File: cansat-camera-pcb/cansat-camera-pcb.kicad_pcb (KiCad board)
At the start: 8 copper layers, 50 x 50 mm, 60 parts, among them IC1 W9825G6JB-6I, IC2 TLV74315PDBVR, J3 Conn_01x05_Socket, J4 Conn_02x10_Odd_Even, J5 Conn_02x10_Odd_Even, J6 OV5640, SW2 SW_Push, U2 AP2112K-3.3, U4 STM32H743ZITx, U6 TLV74328PDBVR, Y1 24MHz

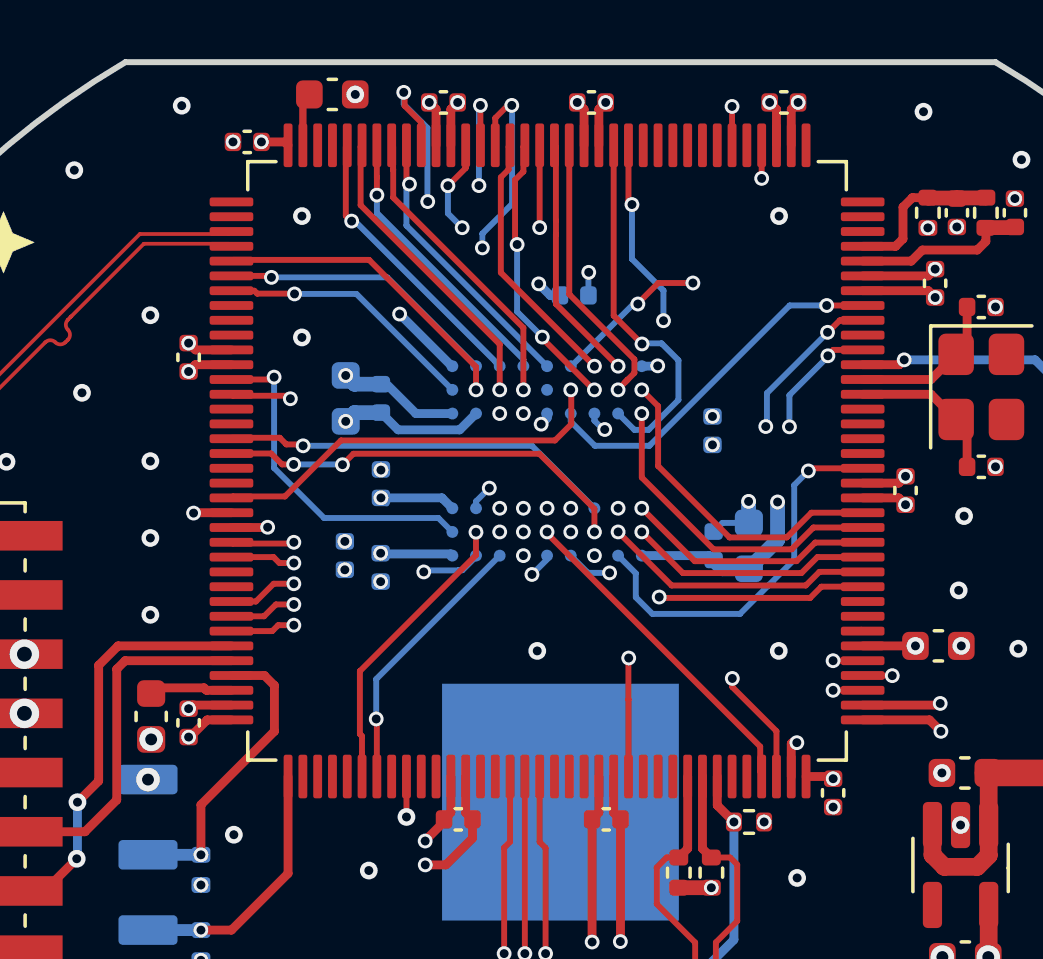
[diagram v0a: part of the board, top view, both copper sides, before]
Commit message: Sdram finish, cleanup
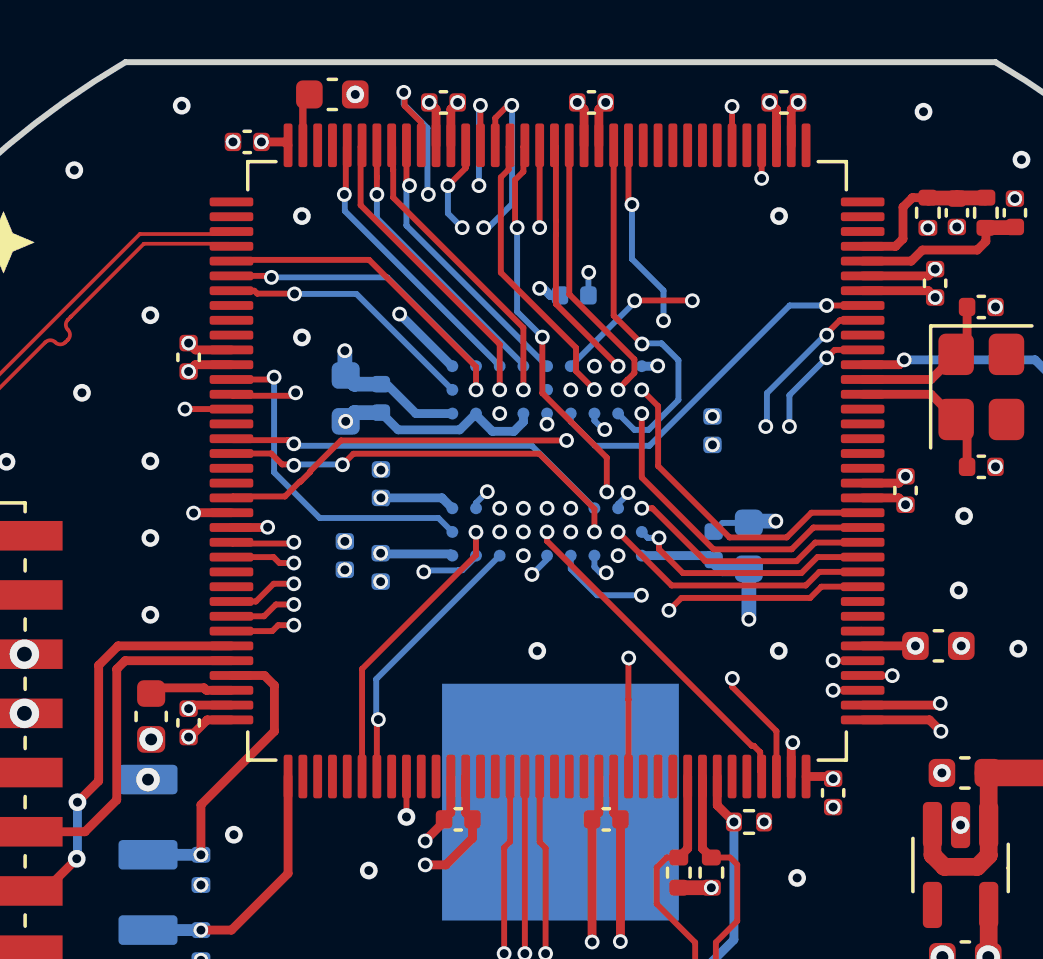
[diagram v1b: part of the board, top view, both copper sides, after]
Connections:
- IC1 pad G1: /FMC_A11 -> /FMC_A12
- IC1 pad G2: /FMC_A10 -> /FMC_A11
- IC1 pad H9: /FMC_AP -> /FMC_A10
- U4 pad 18: /FMC_AP -> unconnected-(U4-PF6-Pad18)
- U4 pad 87: unconnected-(U4-PG2-Pad87) -> /FMC_A12
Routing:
- net /FMC_A12: track 0.00 -> 16.0 mm, vias 0 -> 2
- net /FMC_AP: track 13.1 -> 0.00 mm, vias 1 -> 0
- net /FMC_A10: track 9.52 -> 16.1 mm, vias 3 -> 4
- net +3.3V: track 66.3 -> 62.4 mm, vias 37 -> 36
- net /FMC_D1: track 11.8 -> 14.0 mm
- net /FMC_SDNWE: track 13.9 -> 15.6 mm
- net /FMC_SDNE0: track 13.1 -> 14.6 mm
- net /FMC_SDNCAS: track 14.3 -> 15.7 mm
- net GND: track 38.7 -> 39.6 mm
- net /FMC_A11: track 8.90 -> 9.69 mm
- net /FMC_A0: track 12.0 -> 12.6 mm
- net /FMC_NBL1: track 23.1 -> 22.6 mm
- net /FMC_SDCLK: track 13.7 -> 13.9 mm, vias 1 -> 2

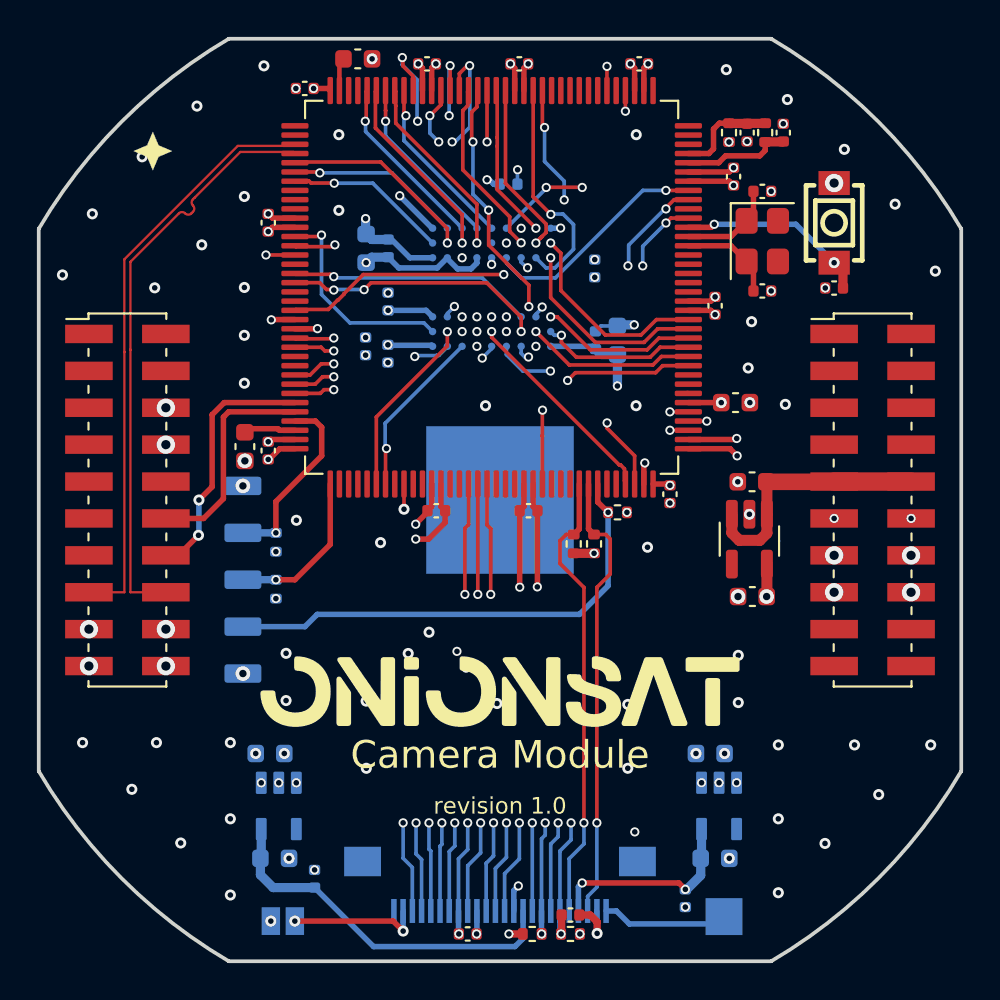
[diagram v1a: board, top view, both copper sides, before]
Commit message: Cleanup finish
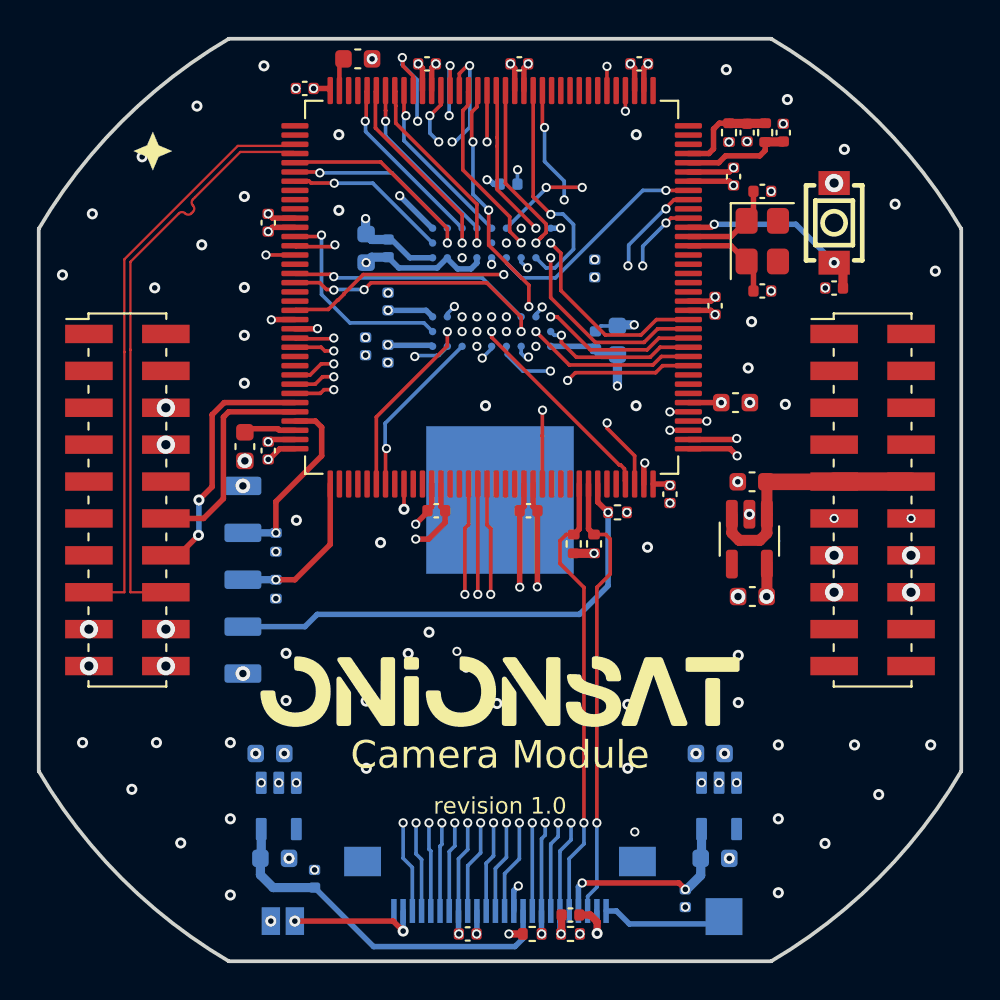
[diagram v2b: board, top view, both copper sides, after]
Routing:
- net /camera/DATA1: track 7.74 -> 7.18 mm
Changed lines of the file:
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@@
 	)
 	(segment
-		(start 68.511012 111.13)
-		(end 68.49 111.13)
-		(width 0.2)
-		(layer "B.Cu")
-		(net 1)
-	)
-	(segment
 		(start 76.672012 112.891)
 		(end 77.199 112.891)
@@
 	)
 	(segment
-		(start 73.19 110.23117)
-		(end 73.19 110.16)
-		(width 0.2)
-		(layer "B.Cu")
-		(net 6)
-	)
-	(segment
 		(start 79.395 119.735)
 		(end 79.1 119.44)
@@
 	)
 	(segment
-		(start 68.05 117.53)
-		(end 67.86 117.34)
-		(width 0.2)
-		(layer "B.Cu")
-		(net 6)
-	)
-	(segment
 		(start 67.86 114.46)
 		(end 66.965 114.46)
@@
 	)
 	(segment
-		(start 73.221013 110.262183)
-		(end 73.19 110.23117)
-		(width 0.2)
-		(layer "B.Cu")
-		(net 6)
-	)
-	(segment
 		(start 69.921012 117.34)
 		(end 67.86 117.34)
@@
 	)
 	(segment
-		(start 73.19 110.23117)
-		(end 73.19 110.16)
-		(width 0.2)
-		(layer "In5.Cu")
-		(net 6)
-	)
-	(segment
-		(start 73.221013 110.262183)
-		(end 73.19 110.23117)
-		(width 0.2)
-		(layer "In5.Cu")
-		(net 6)
-	)
-	(segment
 		(start 73.472012 117.641057)
 		(end 73.472012 117.691)
@@
 	)
 	(segment
-		(start 84.087388 121.793876)
-		(end 84.134512 121.841)
-		(width 0.2)
-		(layer "F.Cu")
-		(net 20)
-	)
-	(segment
 		(start 84.134512 124.841)
 		(end 86.392 124.841)
@@
 	)
 	(segment
-		(start 72.22 126.751488)
-		(end 72.222012 126.7535)
-		(width 0.2)
-		(layer "F.Cu")
-		(net 48)
-	)
-	(segment
 		(start 72.022012 129.157232)
 		(end 72.022012 132.736)
@@
 	)
 	(segment
-		(start 62.8045 150.443)
-		(end 62.8045 151)
-		(width 0.3)
-		(layer "B.Cu")
-		(net 54)
-	)
-	(segment
 		(start 85.669 150.597)
 		(end 80.935 150.597)
@@
 		(net 56)
 	)
-	(segment
-		(start 84.132512 123.839)
-		(end 84.134512 123.841)
-		(width 0.2)
-		(layer "F.Cu")
-		(net 56)
-	)
 	(via
 		(at 71.475 145.118)
@@
 	)
 	(segment
-		(start 69.214319 119.784319)
-		(end 69.214319 119.812633)
-		(width 0.2)
-		(layer "In2.Cu")
-		(net 69)
-	)
-	(segment
 		(start 68.03 113.79)
 		(end 64.977057 113.79)
@@
 	)
 	(segment
-		(start 69.214319 119.812633)
-		(end 69.243954 119.842268)
-		(width 0.2)
-		(layer "In2.Cu")
-		(net 69)
-	)
-	(segment
 		(start 68.64 114.4)
 		(end 68.03 113.79)
@@
 	)
 	(segment
-		(start 69.243954 119.842268)
-		(end 69.305765 119.842268)
-		(width 0.2)
-		(layer "In2.Cu")
-		(net 69)
-	)
-	(segment
 		(start 69.305765 119.842268)
 		(end 69.303856 119.840359)
@@
 	)
 	(segment
-		(start 82.876003 112.606003)
-		(end 82.92 112.606003)
-		(width 0.2)
-		(layer "F.Cu")
-		(net 81)
-	)
-	(segment
 		(start 82.92 112.606003)
 		(end 83.185003 112.341)
@@
 	)
 	(segment
-		(start 75.49 117.14)
-		(end 75.49 116.95)
-		(width 0.2)
-		(layer "B.Cu")
-		(net 84)
-	)
-	(segment
 		(start 76.121012 117.919232)
 		(end 76.423012 118.221232)
@@
 	)
 	(segment
-		(start 75.071 113.691)
-		(end 75.072012 113.691)
-		(width 0.2)
-		(layer "F.Cu")
-		(net 85)
-	)
-	(segment
 		(start 71.91 106.511836)
 		(end 72.173012 106.248824)
@@
 	)
 	(segment
-		(start 69.46 107.21)
-		(end 69.43 107.18)
-		(width 0.2)
-		(layer "B.Cu")
-		(net 97)
-	)
-	(segment
 		(start 68.63 104.04)
 		(end 68.63 103.64)
@@
 	)
 	(segment
-		(start 74.272012 113.691)
-		(end 74.29 113.708988)
-		(width 0.2)
-		(layer "F.Cu")
-		(net 99)
-	)
-	(segment
 		(start 74.13027 115.4)
 		(end 66.51 115.4)
@@
 	)
 	(segment
-		(start 64.85 116.24)
-		(end 64.878806 116.24)
-		(width 0.2)
-		(layer "B.Cu")
-		(net 142)
-	)
-	(segment
 		(start 64.908806 116.21)
 		(end 66.55 116.21)
@@
 	)
 	(segment
-		(start 64.878806 116.24)
-		(end 64.908806 116.21)
-		(width 0.2)
-		(layer "B.Cu")
-		(net 142)
-	)
-	(segment
 		(start 66.55 116.21)
 		(end 66.56 116.22)
@@
 	)
 	(segment
-		(start 64.848474 115.512706)
-		(end 64.880962 115.512706)
-		(width 0.2)
-		(layer "B.Cu")
-		(net 143)
-	)
-	(segment
 		(start 64.880962 115.512706)
 		(end 64.949256 115.581)
@@
 	)
 	(segment
-		(start 57.28378 111.32214)
-		(end 57.369989 111.235932)
-		(width 0.1262)
-		(layer "F.Cu")
-		(net 154)
-	)
-	(segment
 		(start 53.8947 119.474)
 		(end 53.8937 119.473)
@@
 	)
 	(segment
-		(start 57.369989 111.235932)
+		(start 57.28378 111.32214)
 		(end 57.397966 111.207956)
 		(width 0.1262)
@@
 		(target_skew_min -0.1)
 		(tuning_mode "diff_pair_skew")
-		(members "2dbd5204-07fa-484e-9b59-9e6cc3ddea21" "3a1ca473-3f2c-4f43-b50d-bd7720170219"
-			"5d351394-5b7d-483b-a3ed-614d40769c99" "61b585f4-9e34-43c9-812e-ac13c45d3f8a"
-			"638743db-7a85-4eae-8c00-d0526a2abb19" "940f68bf-92de-41b3-aa72-8fac11707541"
-			"cdccc0d4-a090-4d7b-942b-60a9b9b19372"
+		(members "3a1ca473-3f2c-4f43-b50d-bd7720170219" "5d351394-5b7d-483b-a3ed-614d40769c99"
+			"61b585f4-9e34-43c9-812e-ac13c45d3f8a" "638743db-7a85-4eae-8c00-d0526a2abb19"
+			"940f68bf-92de-41b3-aa72-8fac11707541" "cdccc0d4-a090-4d7b-942b-60a9b9b19372"
 		)
 	)
